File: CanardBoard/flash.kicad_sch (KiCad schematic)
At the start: 4 parts, among them U3 GD5F1GM7UEYIGR

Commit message: more schematic
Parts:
- U3: footprint SON127P800X600X80-9N-D -> canardboard:GD5F1GM7UEYIGR
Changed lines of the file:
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@@
 			)
 		)
-		(property "Footprint" "SON127P800X600X80-9N-D"
+		(property "Footprint" "canardboard:GD5F1GM7UEYIGR"
 			(at 213.36 196.52 0)
 			(effects

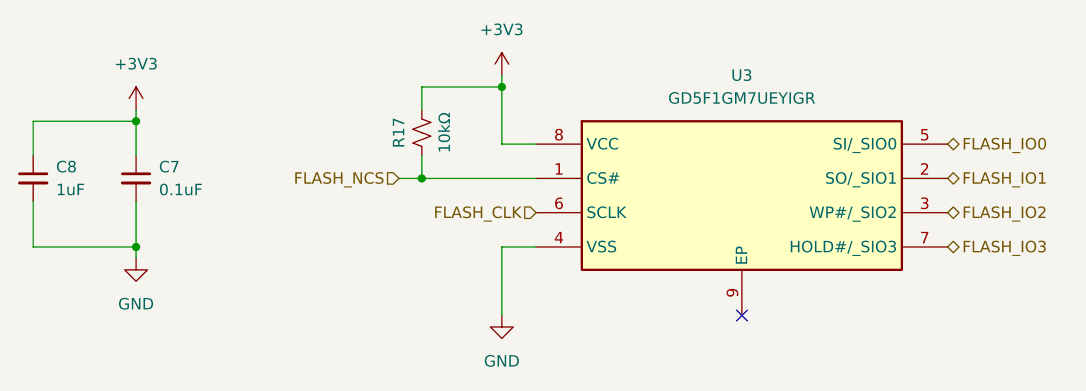
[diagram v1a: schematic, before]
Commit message: more schematic work
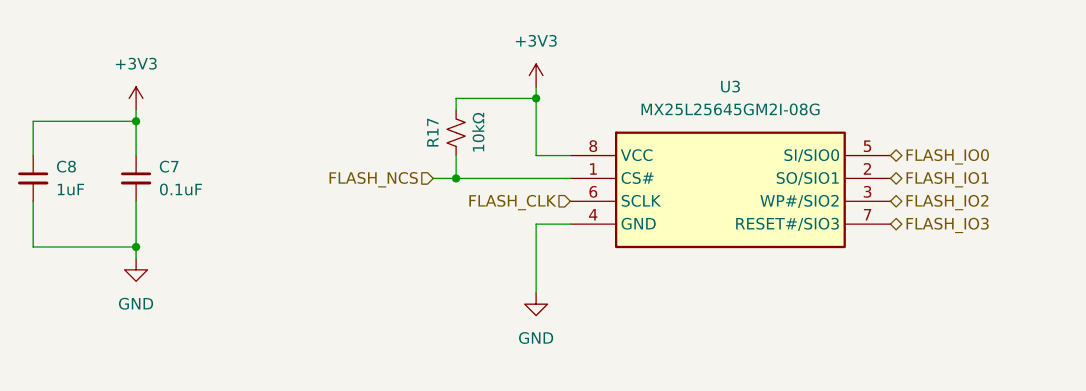
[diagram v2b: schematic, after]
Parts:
- removed U3: GD5F1GM7UEYIGR, canardboard:GD5F1GM7UEYIGR, symbol canardboard:GD5F1GM7UEYIGR
- added U3: MX25L25645GM2I-08G, SOIC127P790X216-8N, symbol canardboard:MX25L25645GM2I-08G
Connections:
- net +3V3: now also U3.8 (VCC)
- net FLASH_CLK: now also U3.6 (SCLK)
- net FLASH_IO0: now also U3.5 (SI/SIO0)
- net FLASH_IO1: now also U3.2 (SO/SIO1)
- net FLASH_IO2: now also U3.3 (WP#/SIO2)
- net FLASH_IO3: now also U3.7 (RESET#/SIO3)
- net FLASH_NCS: now also U3.1 (CS#)
- net GND: now also U3.4 (GND)
- no-connect marks 1 -> 0
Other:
- moved on the sheet: R17

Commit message: mag
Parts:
- U3: footprint SOIC127P790X216-8N -> (none)
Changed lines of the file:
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@@
 			)
 		)
-		(property "Footprint" "SOIC127P790X216-8N"
+		(property "Footprint" ""
 			(at 191.77 191.44 0)
 			(effects

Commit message: AD Breakout interface
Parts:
- U3: footprint (none) -> SOIC127P790X216-8N
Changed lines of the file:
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@@
 			)
 		)
-		(property "Footprint" ""
+		(property "Footprint" "SOIC127P790X216-8N"
 			(at 191.77 191.44 0)
 			(effects

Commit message: work
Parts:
- C7, C8: footprint Capacitor_SMD:C_0805_2012Metric_Pad1.18x1.45mm_HandSolder -> Capacitor_SMD:C_0402_1005Metric
- R17: footprint Resistor_SMD:R_0805_2012Metric_Pad1.20x1.40mm_HandSolder -> Resistor_SMD:R_0402_1005Metric
- U3: footprint SOIC127P790X216-8N -> canardboard:MX25L25645GM2I-08G
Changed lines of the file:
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@@
 			)
 		)
-		(property "Footprint" "SOIC127P790X216-8N"
+		(property "Footprint" "canardboard:MX25L25645GM2I-08G"
 			(at 191.77 191.44 0)
 			(effects
@@
 			)
 		)
-		(property "Footprint" "Capacitor_SMD:C_0805_2012Metric_Pad1.18x1.45mm_HandSolder"
+		(property "Footprint" "Capacitor_SMD:C_0402_1005Metric"
 			(at 92.71 99.06 0)
 			(effects
@@
 			)
 		)
-		(property "Footprint" "Capacitor_SMD:C_0805_2012Metric_Pad1.18x1.45mm_HandSolder"
+		(property "Footprint" "Capacitor_SMD:C_0402_1005Metric"
 			(at 104.14 99.06 0)
 			(effects
@@
 			)
 		)
-		(property "Footprint" "Resistor_SMD:R_0805_2012Metric_Pad1.20x1.40mm_HandSolder"
+		(property "Footprint" "Resistor_SMD:R_0402_1005Metric"
 			(at 139.7 93.98 0)
 			(effects
